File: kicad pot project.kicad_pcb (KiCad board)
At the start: 2 copper layers, 7 parts, among them P1 POT1, P2 POT2, P3 POT3, P4 POT4, P5 POT5, P6 POT6

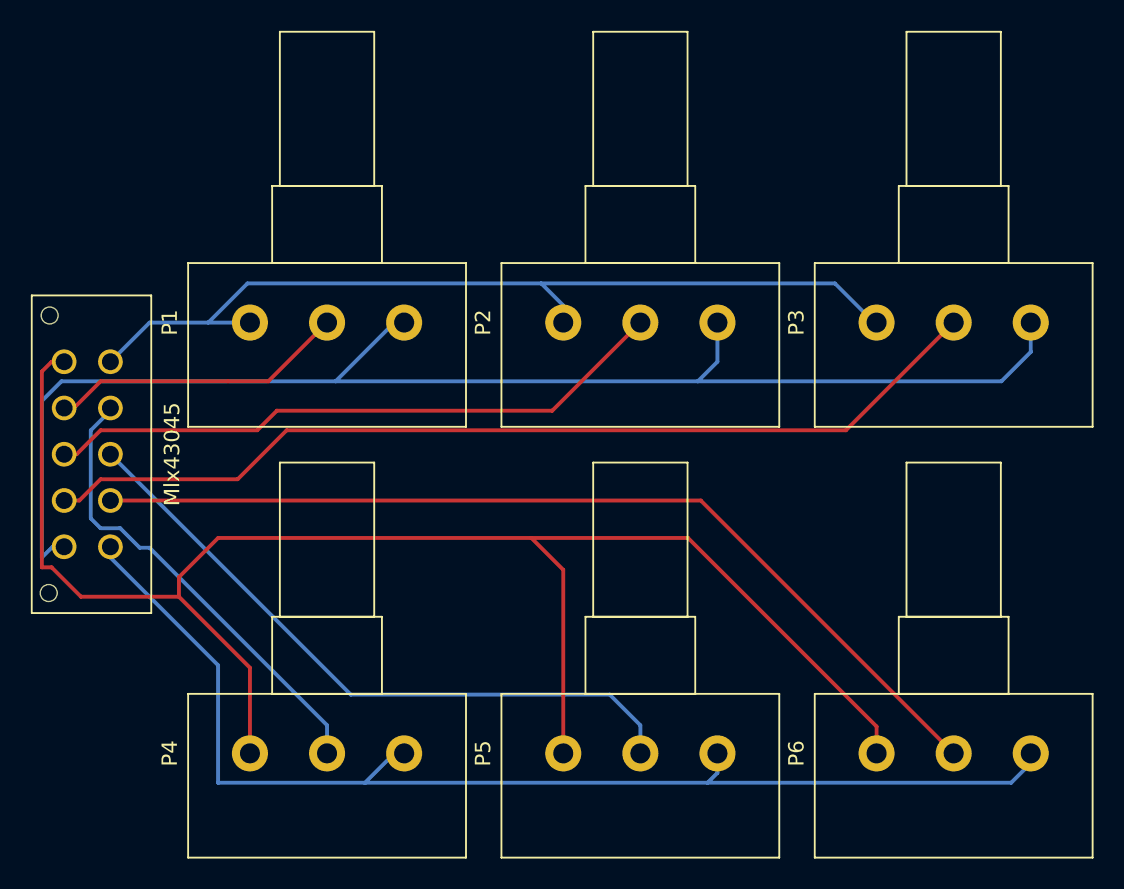
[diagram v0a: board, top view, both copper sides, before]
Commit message: Add files via upload
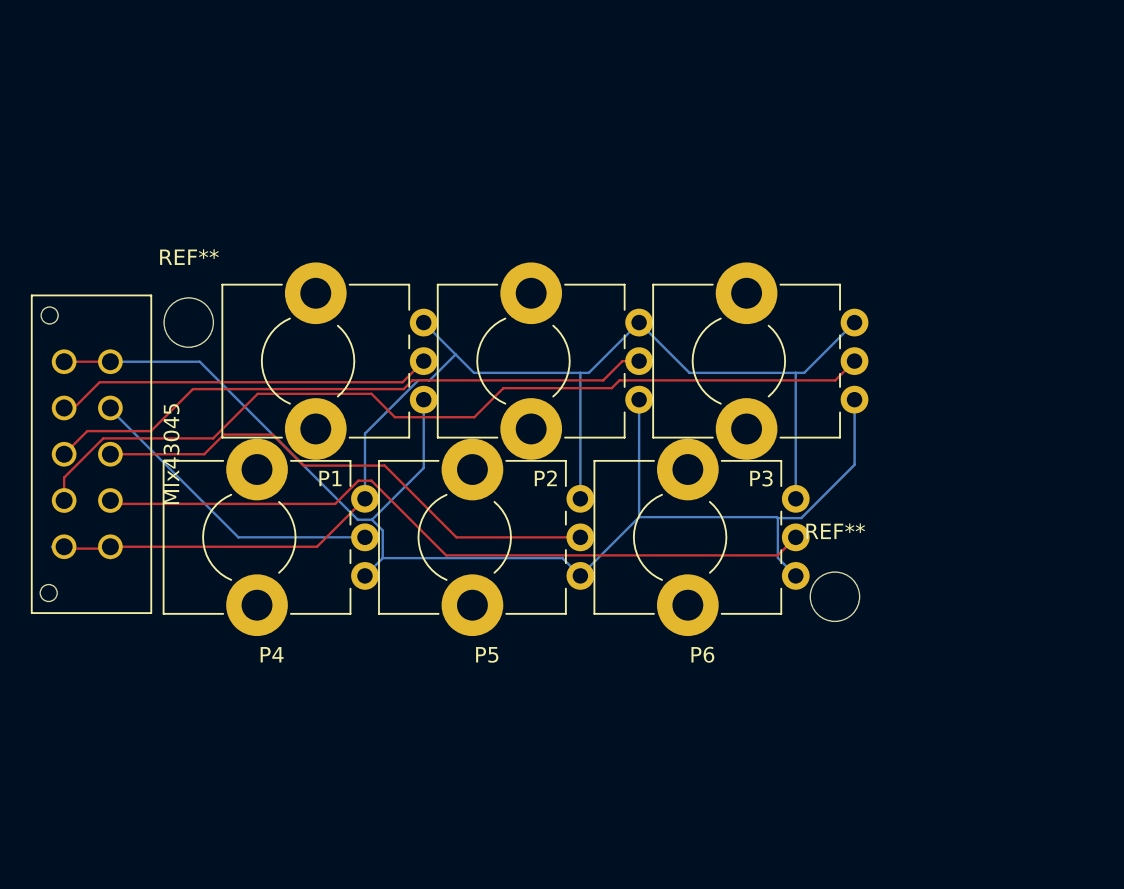
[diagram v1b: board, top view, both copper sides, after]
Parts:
- added REF**: MountingHole_3.2mm_M3, Mounting_Holes:MountingHole_3.2mm_M3, F.Cu at (175.3, 106.7)
- added REF**: MountingHole_3.2mm_M3, Mounting_Holes:MountingHole_3.2mm_M3, F.Cu at (133.3, 88.9)
- P1, P2, P3, P4, P5, P6: footprint Potentiometers:Potentiometer_Alps_RK163_Single_Vertical -> Potentiometers:Potentiometer_Alps_RK09K_Horizontal
- moved P6 22.5 mm to (172.7, 100.3), turned to 180 degrees
- moved P5 18.8 mm to (158.8, 100.3), turned to 180 degrees
- moved P4 16.7 mm to (144.8, 100.3), turned to 180 degrees
- moved P3 11.4 mm to (176.5, 88.9), turned to 180 degrees
- moved P2 5.08 mm to (162.6, 88.9), turned to 180 degrees
- moved P1 1.27 mm to (148.6, 88.9), turned to 180 degrees
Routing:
- net GND: track 167.4 -> 84.4 mm
- net +3V3: track 165.1 -> 88.0 mm
- net AO6: track 61.5 -> 47.7 mm
- net AO4: track 30.4 -> 20.1 mm
- net AO5: track 43.8 -> 33.8 mm
- net AO3: track 62.5 -> 57.1 mm
- net AO1: track 19.4 -> 24.6 mm
- net AO2: track 40.9 -> 39.8 mm
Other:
- net class Default: clearance 0.2 -> 0.1524; trace_width 0.25 -> 0.1524; via_dia 0.6 -> 0.5842; via_drill 0.4 -> 0.3302
- rule pad_to_mask_clearance: 0.2 -> 0.0508
- rule trace_clearance: 0.2 -> 0.1524
- rule trace_min: 0.006 -> 0.1524
- rule via_min_drill: 0.013 -> 0.3302
- rule via_min_size: 0.027 -> 0.5842
